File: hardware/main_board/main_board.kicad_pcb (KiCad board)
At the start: 2 copper layers, 95.3 x 71.6 mm, 85 parts, among them IC1 E22-900M22S, IC2 INA226AIDGST, IC3 INA226AIDGST, IC4 TPS2121RUXT, IC5 TP5000-QFN16, J1 power swith, J2 I2C External Modules, J3 Solar panel, J5 Battary over BMS, J6 USB4105-GF-A-060, U1 ESP32-C3-WROOM-02, U2 DS3231SN, U4 TPS631000DRLR, U5 PCA9536DR

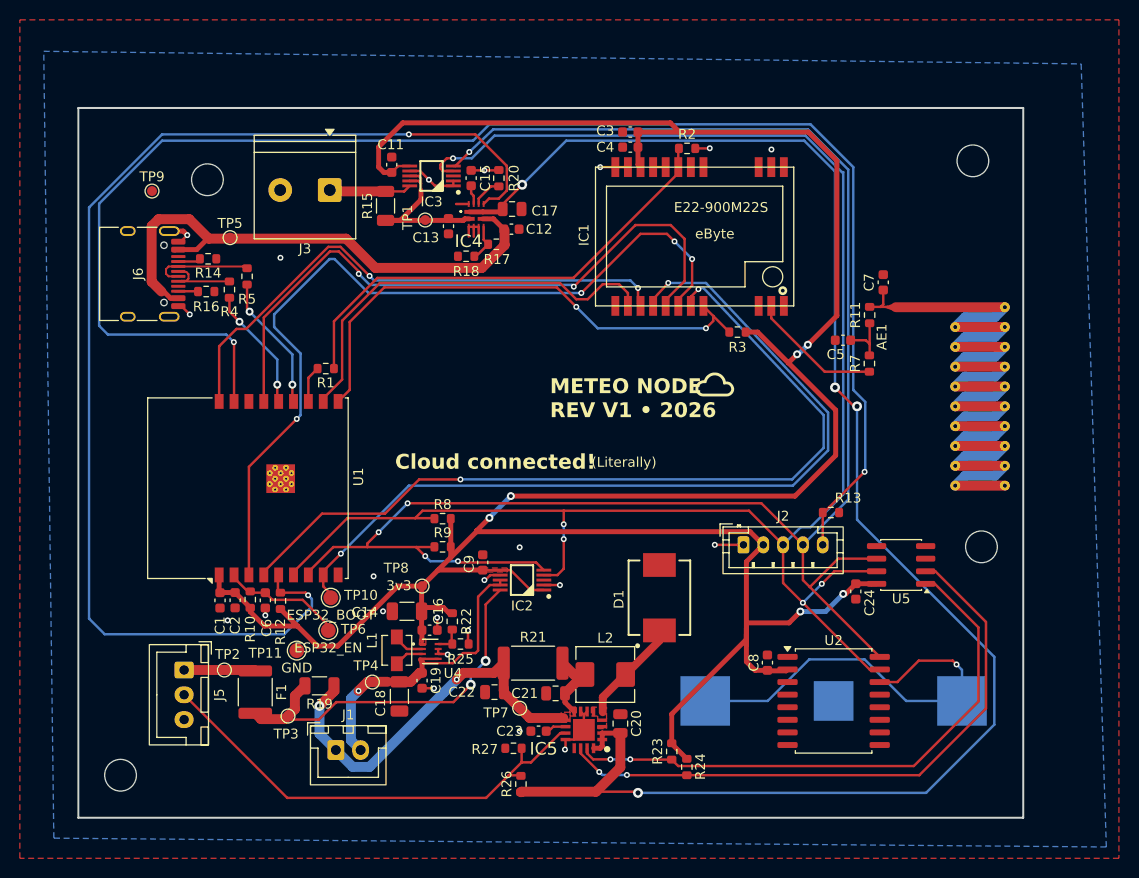
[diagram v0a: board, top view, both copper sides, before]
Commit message: hw v1 resize board
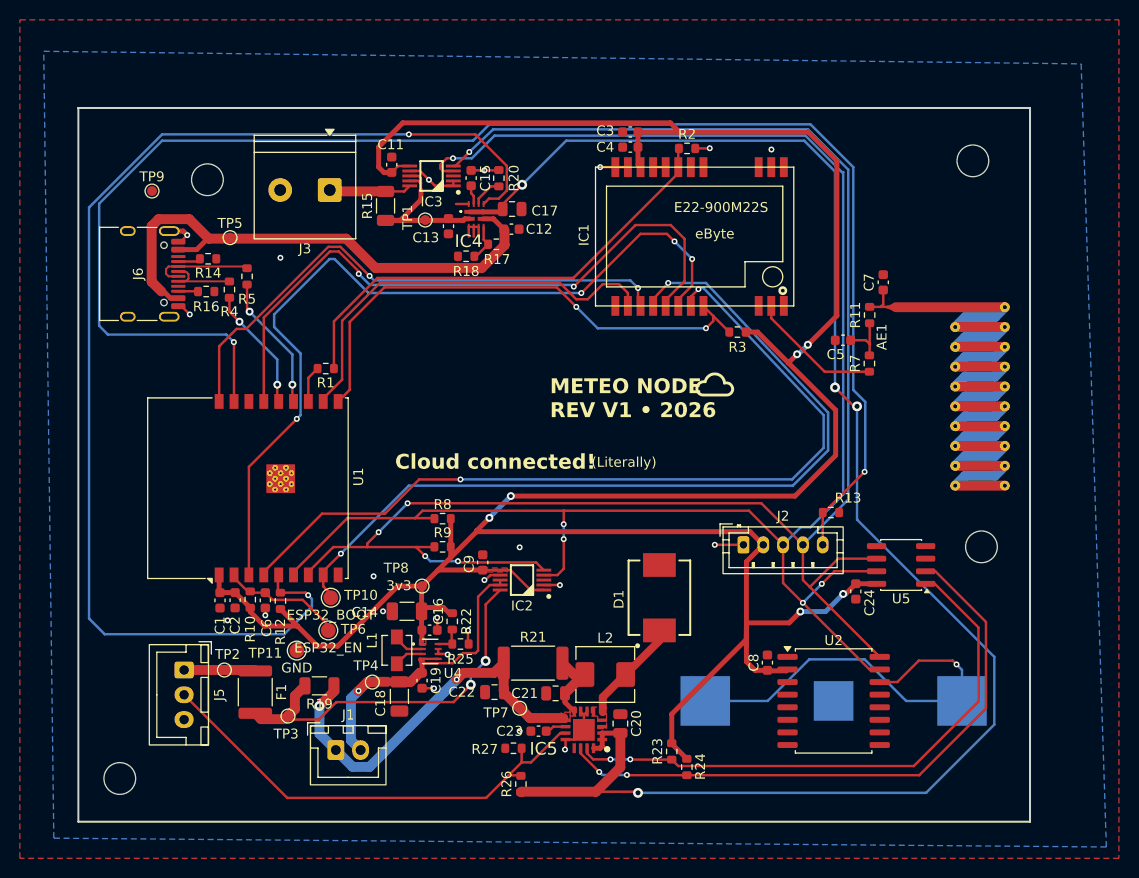
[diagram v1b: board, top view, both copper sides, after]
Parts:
- moved REF4 0.34 mm to (106.0, 132.8)
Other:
- board size 95.3 x 71.6 mm -> 96 x 72 mm
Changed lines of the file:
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@@
 	(footprint "MountingHole:MountingHole_3.2mm_M3"
 		(layer "F.Cu")
-		(at 106.045 132.461)
+		(at 105.9688 132.7912)
 		(descr "Mounting Hole 3.2mm, M3, no annular, generated by kicad-footprint-generator mountinghole.py")
 		(tags "mountinghole M3")
@@
 	(gr_rect
 		(start 101.7884 65.151)
-		(end 197.104 136.7524)
+		(end 197.7884 137.151)
 		(stroke
 			(width 0.2)
@@
 	)
 	(gr_text "Якщо читаєш це - поверни назад у корпус."
-		(at 143.764 135.128 0)
+		(at 144.2212 135.7376 0)
 		(layer "B.SilkS")
 		(effects
